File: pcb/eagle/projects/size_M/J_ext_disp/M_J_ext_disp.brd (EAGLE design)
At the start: 11 parts, among them J1 SSD_1306_STM32_OLED

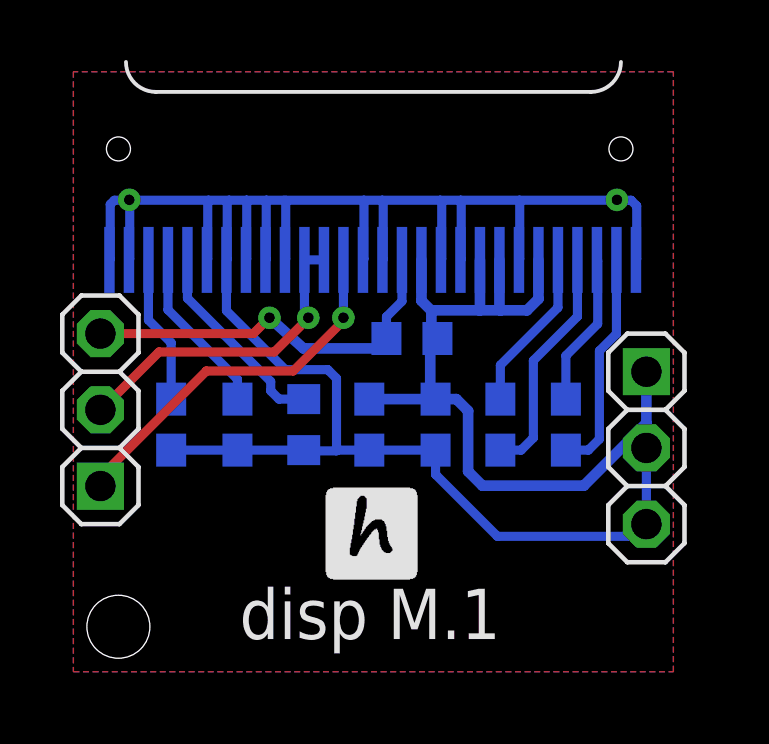
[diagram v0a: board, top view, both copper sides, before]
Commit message: PCB M.1
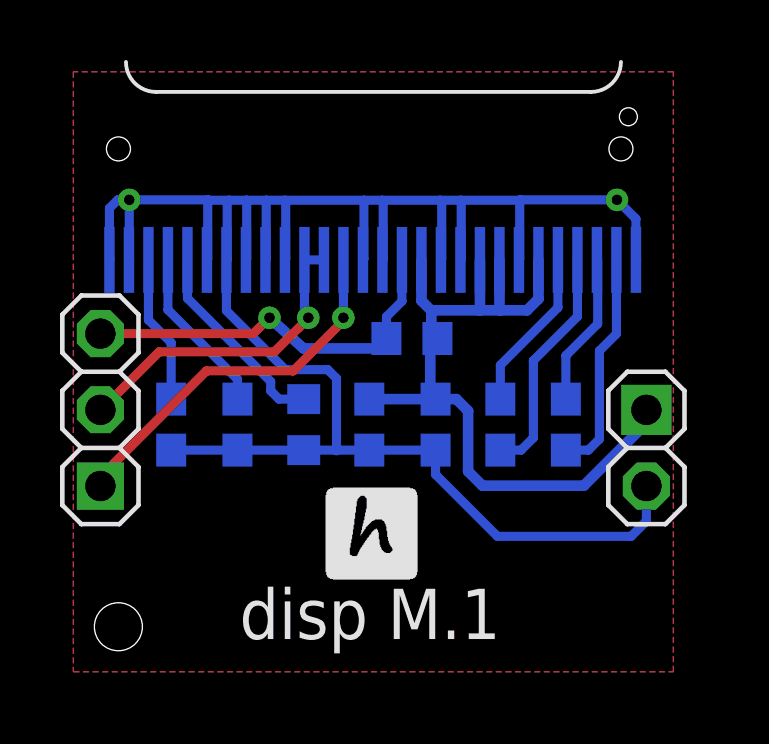
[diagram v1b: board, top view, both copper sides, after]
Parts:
- removed JP2: (no value), pinhead2:1X03
- added I.J2: (no value), pinhead2:1X02
- renumbered H.C1 to J.C1, H.C2 to J.C2, H.C3 to J.C3, H.C4 to J.C4, H.C5 to J.C5, H.C6 to J.C6, H.R1 to J.R1, H.R2 to J.R2, J1 to I.J3, JP1 to J.J1
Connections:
- net GND: now also I.J2.2; no longer JP2.2
- net VDD: now also I.J2.1; no longer JP2.1
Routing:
- net GND: track 72.2 -> 70.9 mm
- net VDD: track 27.6 -> 26.4 mm

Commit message: updated PCBs for version 2
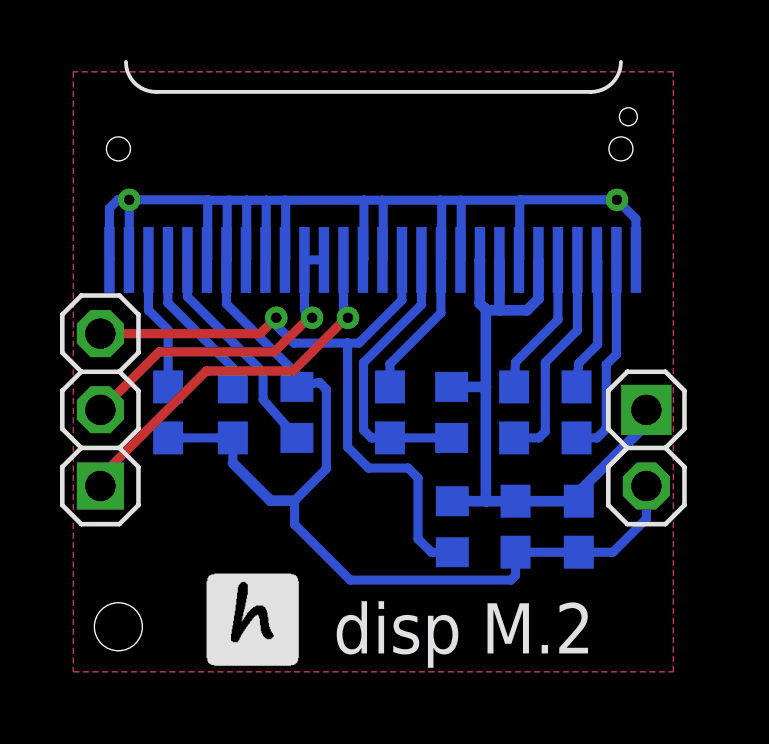
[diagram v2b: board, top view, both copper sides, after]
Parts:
- added J.C7: 2u2, rcl:C0603
- added J.R3: 2k2, rcl:R0603
- moved J.R2 6.42 mm to (13.1, 5.33), turned to 90 degrees
- moved J.C6 5.95 mm to (15.2, 5.33)
- moved J.C5 5.86 mm to (17.3, 5.33)
- moved J.C4 0.61 mm to (15.2, 9.14)
- moved J.C1 0.54 mm to (17.3, 9.14)
- moved J.R1 0.47 mm to (7.95, 9.14), turned to 270 degrees
- moved J.C2 0.43 mm to (5.82, 9.14)
- moved J.C3 0.42 mm to (3.66, 9.14)
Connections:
- new net N$2: I.J3.P$12, J.C7.2, J.R3.2
- net GND: now also J.C7.1
- net VDD: now also J.R3.1; no longer I.J3.P$12
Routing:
- net N$2: track 0.00 -> 9.57 mm
- net PA7: track 13.1 -> 22.3 mm
- net GND: track 70.9 -> 79.9 mm
- net VDD: track 26.4 -> 22.6 mm
- net N$7: track 7.82 -> 6.89 mm
- net N$1: track 6.73 -> 7.40 mm
- net N$10: track 5.44 -> 4.82 mm
- net N$8: track 5.09 -> 4.51 mm
- net N$9: track 7.81 -> 7.29 mm
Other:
- board text added: "disp M.2"
- board text removed: "disp M.1"
